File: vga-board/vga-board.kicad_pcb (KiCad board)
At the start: 2 copper layers, 105.4 x 61.6 mm, 24 parts, among them J1 EXP, J2 EXP, J3 Conn_02x05_Odd_Even, U1 XC95144XL-TQ100, U2 IS61C5128AL-10TLI, X1 50MHz

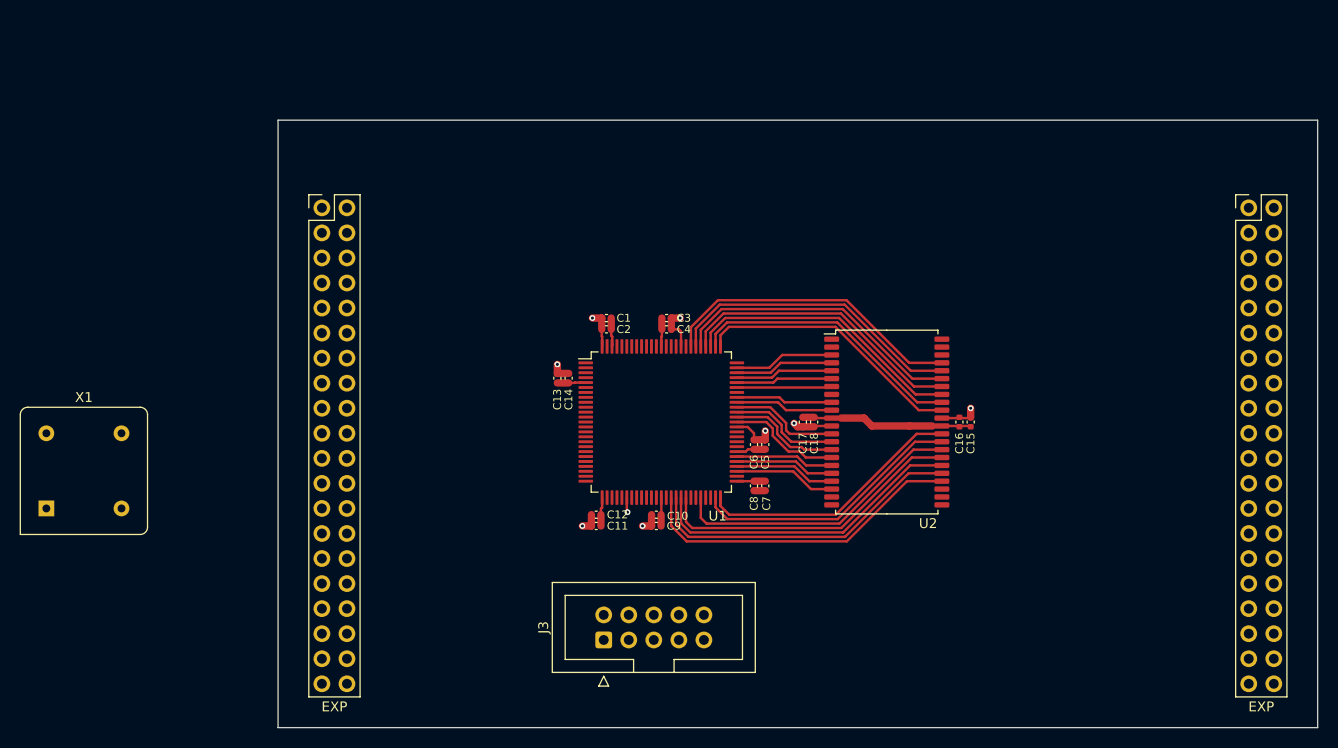
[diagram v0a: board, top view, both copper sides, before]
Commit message: more vga board routing
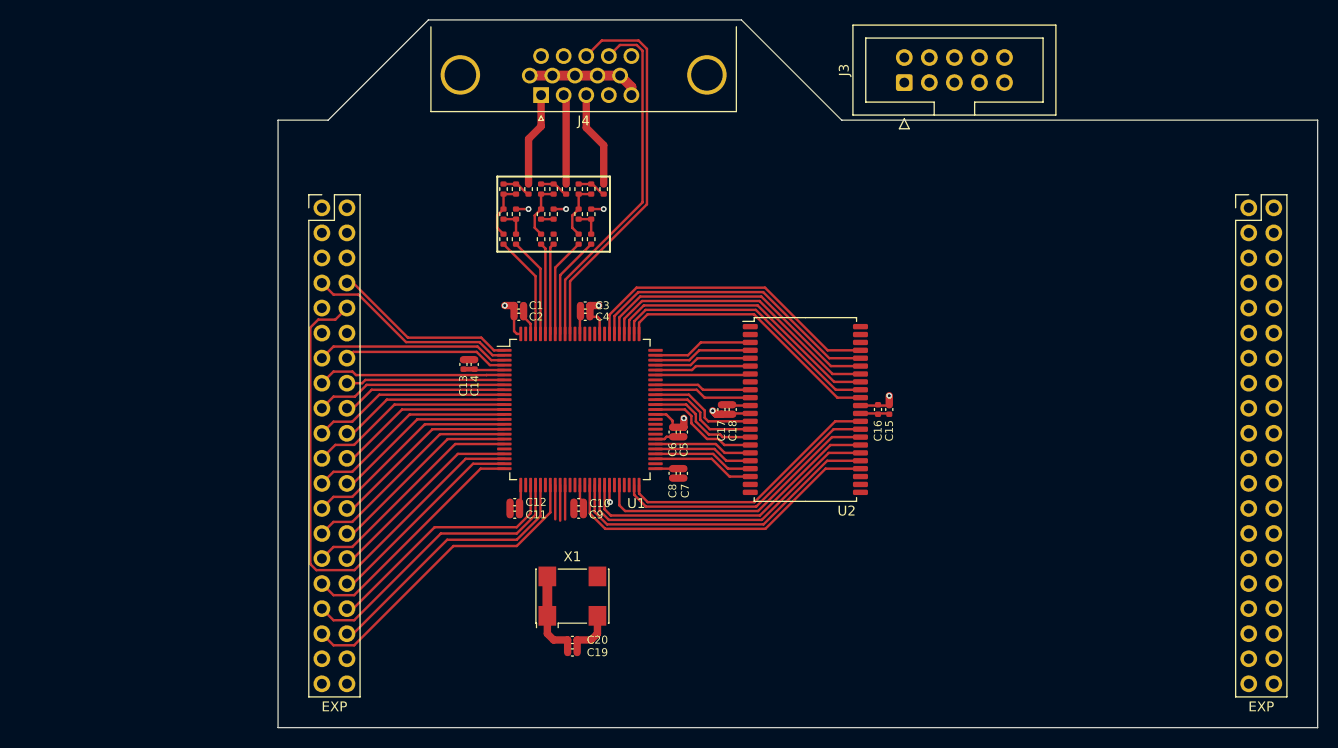
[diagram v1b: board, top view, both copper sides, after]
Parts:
- added C19: 100n, Capacitor_SMD:C_0402_1005Metric, F.Cu at (71.1, 111.1)
- added C20: 10n, Capacitor_SMD:C_0402_1005Metric, F.Cu at (71.1, 109.9)
- added J4: DB15_Female_HighDensity, Connector_Dsub:DSUB-15-HD_Female_Horizontal_P2.29x1.98mm_EdgePinOffset3.03mm_Housed_MountingHolesOffset4.94mm, F.Cu at (67.9, 54.6)
- added R1: 560R, Resistor_SMD:R_0402_1005Metric, F.Cu at (64.1, 69.2)
- added R10: 560R, Resistor_SMD:R_0402_1005Metric, F.Cu at (67.9, 64.1)
- added R11: 560R, Resistor_SMD:R_0402_1005Metric, F.Cu at (67.9, 66.7)
- added R12: 560R, Resistor_SMD:R_0402_1005Metric, F.Cu at (69.2, 66.7)
- added R13: 47R, Resistor_SMD:R_0402_1005Metric, F.Cu at (70.5, 64.1)
- added R14: 560R, Resistor_SMD:R_0402_1005Metric, F.Cu at (69.2, 64.1)
- added R15: 560R, Resistor_SMD:R_0402_1005Metric, F.Cu at (71.8, 69.2)
- added R16: 560R, Resistor_SMD:R_0402_1005Metric, F.Cu at (73.0, 69.2)
- added R17: 560R, Resistor_SMD:R_0402_1005Metric, F.Cu at (71.8, 64.1)
- added R18: 560R, Resistor_SMD:R_0402_1005Metric, F.Cu at (71.8, 66.7)
- added R19: 560R, Resistor_SMD:R_0402_1005Metric, F.Cu at (73.0, 66.7)
- added R2: 560R, Resistor_SMD:R_0402_1005Metric, F.Cu at (65.4, 69.2)
- added R20: 47R, Resistor_SMD:R_0402_1005Metric, F.Cu at (74.3, 64.1)
- added R21: 560R, Resistor_SMD:R_0402_1005Metric, F.Cu at (73.0, 64.1)
- added R3: 560R, Resistor_SMD:R_0402_1005Metric, F.Cu at (64.1, 64.1)
- added R4: 560R, Resistor_SMD:R_0402_1005Metric, F.Cu at (64.1, 66.7)
- added R5: 560R, Resistor_SMD:R_0402_1005Metric, F.Cu at (65.4, 66.7)
- added R6: 560R, Resistor_SMD:R_0402_1005Metric, F.Cu at (65.4, 64.1)
- added R7: 47R, Resistor_SMD:R_0402_1005Metric, F.Cu at (66.7, 64.1)
- added R8: 560R, Resistor_SMD:R_0402_1005Metric, F.Cu at (67.9, 69.2)
- added R9: 560R, Resistor_SMD:R_0402_1005Metric, F.Cu at (69.2, 69.2)
- X1: value 50MHz -> ABLNO; footprint Oscillator:Oscillator_DIP-8 -> Oscillator:Oscillator_SMD_Abracon_ASV-4Pin_7.0x5.1mm
- moved J3 64.2 mm to (104.8, 53.3)
- moved X1 54.1 mm to (71.1, 105.4)
- moved C13 9.63 mm to (60.1, 81.9)
- moved C14 9.63 mm to (61.2, 81.9)
- moved C1 8.98 mm to (65.7, 75.9)
- moved C2 8.98 mm to (65.7, 77.1)
- moved C15 8.35 mm to (103.3, 86.5)
- moved C16 8.35 mm to (102.1, 86.5)
- moved C17 8.35 mm to (86.2, 86.5)
- moved C18 8.35 mm to (87.4, 86.5)
- moved C5 8.35 mm to (82.4, 88.8)
- moved C6 8.35 mm to (81.3, 88.8)
- moved U1 8.35 mm to (71.9, 86.5)
- moved U2 8.35 mm to (94.7, 86.5)
- moved C12 8.35 mm to (65.3, 95.9)
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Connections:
- U1 pad 1: A0 -> !RESET
- U1 pad 10: Net-(U1-Pad10) -> A6
- U1 pad 11: A8 -> A7
- U1 pad 12: A9 -> A8
- U1 pad 13: A10 -> A9
- U1 pad 14: A11 -> A10
- U1 pad 15: A12 -> A11
- U1 pad 16: A13 -> A12
- U1 pad 17: A14 -> A13
- U1 pad 18: A15 -> A14
- U1 pad 19: Net-(U1-Pad19) -> A15
- U1 pad 2: A1 -> R!W
- U1 pad 20: Net-(U1-Pad20) -> D0
- U1 pad 22: CLK_V -> D1
- U1 pad 24: D0 -> D3
- U1 pad 25: D1 -> D2
- U1 pad 27: D2 -> CLK_V
- U1 pad 28: D3 -> D5
- U1 pad 3: A2 -> A0
- U1 pad 30: D5 -> D7
- U1 pad 33: D7 -> Net-(U1-Pad33)
- U1 pad 4: A3 -> A1
- U1 pad 6: A4 -> A2
- U1 pad 7: A5 -> A3
- U1 pad 8: A6 -> A4
- U1 pad 9: A7 -> A5
- U1 pad 90: Net-(U1-Pad90) -> HSYNC
- U1 pad 91: Net-(U1-Pad91) -> VSYNC
- U1 pad 92: Net-(U1-Pad92) -> B0
- U1 pad 93: Net-(U1-Pad93) -> B1
- U1 pad 94: Net-(U1-Pad94) -> G0
- U1 pad 95: Net-(U1-Pad95) -> G1
- U1 pad 96: Net-(U1-Pad96) -> R0
- U1 pad 97: Net-(U1-Pad97) -> R1
- X1 pad 1: Net-(X1-Pad1) -> +3V3
- X1 pad 4: GND -> +3V3
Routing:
- net CLK: track 0.00 -> 53.1 mm
- net HSYNC: track 0.00 -> 39.3 mm
- net VSYNC: track 0.00 -> 36.1 mm
- net D6: track 0.00 -> 32.0 mm
- net D4: track 0.00 -> 29.6 mm
- net D7: track 0.00 -> 27.7 mm
- net D5: track 0.00 -> 25.5 mm
- net D2: track 0.00 -> 24.3 mm
- net D0: track 0.00 -> 23.3 mm
- net A14: track 0.00 -> 22.7 mm
- net A12: track 0.00 -> 22.0 mm
- net R!W: track 0.00 -> 21.5 mm
- net A10: track 0.00 -> 21.4 mm
- net D3: track 0.00 -> 21.0 mm
- net A8: track 0.00 -> 20.8 mm
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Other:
- board size 105.4 x 61.6 mm -> 105.4 x 71.8 mm
